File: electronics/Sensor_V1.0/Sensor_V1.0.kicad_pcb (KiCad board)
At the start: 2 copper layers, 45.9 x 25.6 mm, 55 parts, among them J1 nuclone_small_left, J2 nuclone_small_right, J5 DevBoardUartInput, Q1 BC846, U1 PPG_sensor, U2 reference_sot23-3, U3 MCP6541

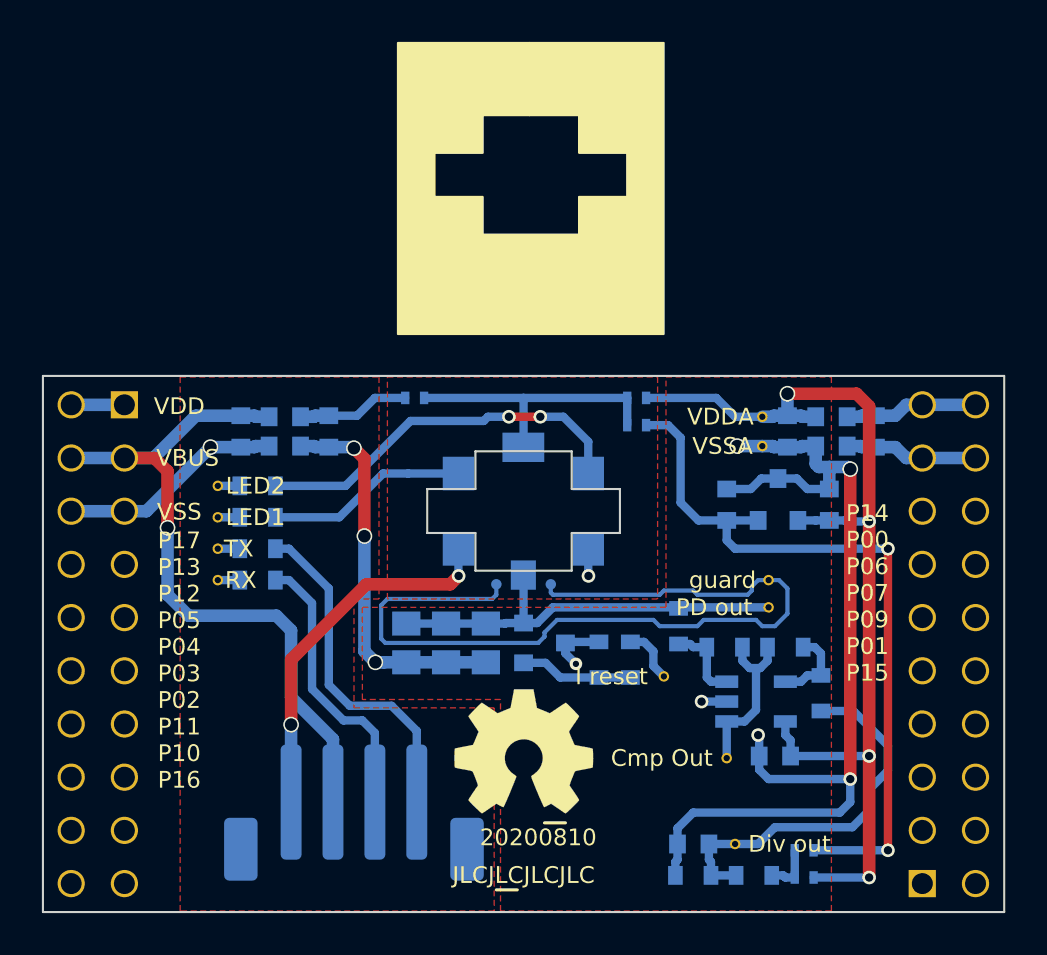
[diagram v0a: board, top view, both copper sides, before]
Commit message: more silk placements
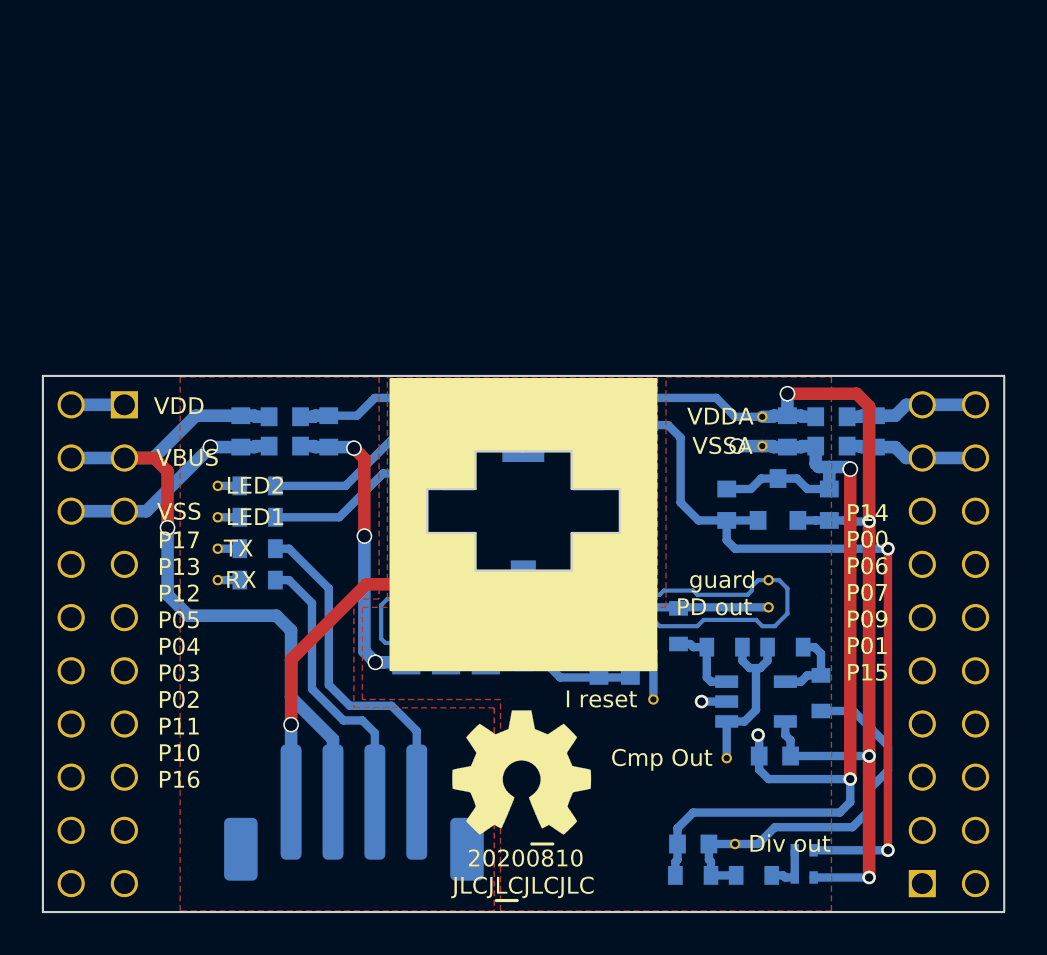
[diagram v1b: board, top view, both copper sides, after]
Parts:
- moved TP12 1.21 mm to (91.3, 89.0)
- moved N2 1.17 mm to (86.0, 96.5)
- moved N1 1.01 mm to (85.0, 92.5)
- moved N3 0.51 mm to (84.3, 98.0)
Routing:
- net /I_reset: track 2.69 -> 3.59 mm
